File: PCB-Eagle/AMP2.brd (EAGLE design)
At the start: 100.4 x 80 mm, 51 parts, among them IC1 LD117AS33TR, IC2 R-78E-0.5, IC3 TL77005ACD, X3 MKDSN1,5/2-5,08

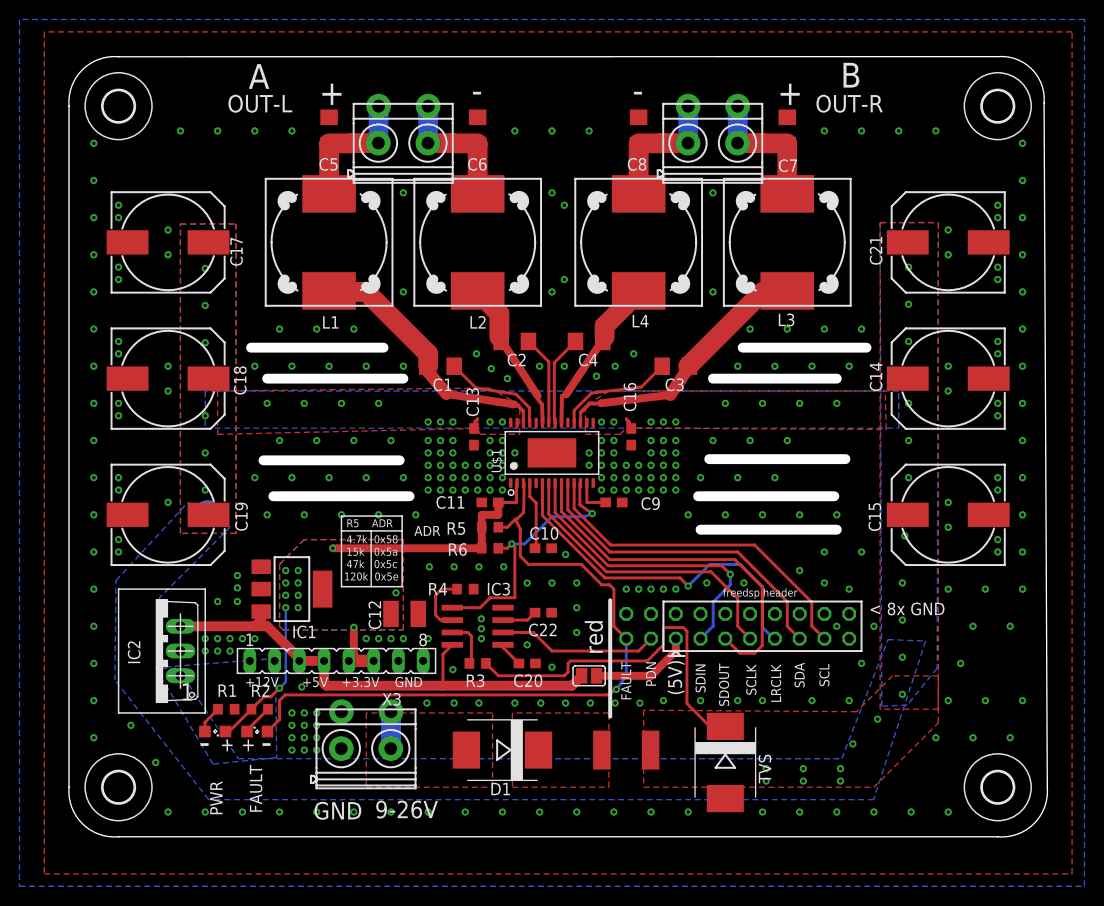
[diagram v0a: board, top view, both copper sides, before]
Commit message: LED 1206.
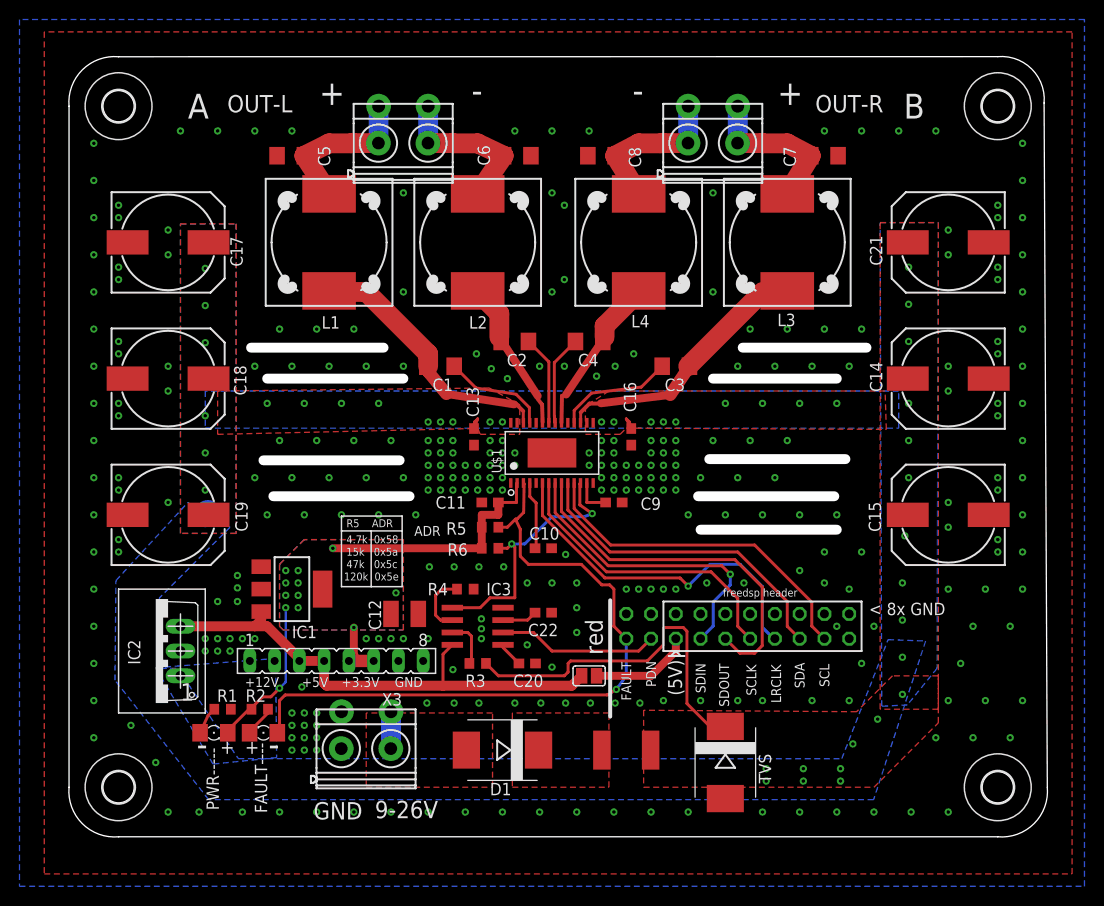
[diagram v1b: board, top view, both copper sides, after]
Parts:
- removed FAULT, PWR: (no value), led:SML0805
- added FAULT----, PWR-----: (no value), led:1206
- R1, R2: value 220 -> 2.2k
- moved C6 4.79 mm to (46.0, 69.8), turned to 0 degrees
- moved C5 4.69 mm to (22.7, 69.8), turned to 180 degrees
- moved C7 4.58 mm to (77.5, 69.8), turned to 0 degrees
- moved C8 4.58 mm to (54.6, 69.8), turned to 180 degrees
- moved R1 0.38 mm to (15.7, 13.1)
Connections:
- net +3V3: now also PWR-----.C; no longer PWR.C
- net ADR/FAULT: now also FAULT----.A; no longer FAULT.A
- net N$13: now also PWR-----.A; no longer PWR.A
- net N$17: now also FAULT----.C; no longer FAULT.C
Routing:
- net N$10: track 14.1 -> 16.6 mm
- net N$1: track 14.0 -> 16.4 mm
- net N$12: track 14.0 -> 16.2 mm
- net N$11: track 14.1 -> 16.2 mm
